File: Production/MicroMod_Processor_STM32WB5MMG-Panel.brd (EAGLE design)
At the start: 199.6 x 83.1 mm, 438 parts, among them J1 MICROMOD-2222, J10 MICROMOD-2222, J11 MICROMOD-2222, J12 MICROMOD-2222, J13 MICROMOD-2222, J14 MICROMOD-2222, J15 MICROMOD-2222, J16 MICROMOD-2222, J2 MICROMOD-2222, J3 MICROMOD-2222, J4 MICROMOD-2222, J5 MICROMOD-2222, J6 MICROMOD-2222, J7 MICROMOD-2222, J8 MICROMOD-2222, J9 MICROMOD-2222, Q1 20V/4.2A/52mΩ/1.4W, Q10 20V/4.2A/52mΩ/1.4W, Q11 20V/4.2A/52mΩ/1.4W, Q12 20V/4.2A/52mΩ/1.4W, Q13 20V/4.2A/52mΩ/1.4W, Q14 20V/4.2A/52mΩ/1.4W, Q15 20V/4.2A/52mΩ/1.4W, Q16 20V/4.2A/52mΩ/1.4W, Q2 20V/4.2A/52mΩ/1.4W, Q3 20V/4.2A/52mΩ/1.4W, Q4 20V/4.2A/52mΩ/1.4W, Q5 20V/4.2A/52mΩ/1.4W, Q6 20V/4.2A/52mΩ/1.4W, Q7 20V/4.2A/52mΩ/1.4W, Q8 20V/4.2A/52mΩ/1.4W, Q9 20V/4.2A/52mΩ/1.4W, U1 STM32WB5MMG, U10 STM32WB5MMG, U11 W25QXX128MBIT-6X5, U12 ESD Diode, U13 STM32WB5MMG, U14 W25QXX128MBIT-6X5, U15 ESD Diode, U16 STM32WB5MMG, U17 W25QXX128MBIT-6X5, U18 ESD Diode, U19 STM32WB5MMG, U2 W25QXX128MBIT-6X5, U20 W25QXX128MBIT-6X5, U21 ESD Diode, U22 STM32WB5MMG, U23 W25QXX128MBIT-6X5, U24 ESD Diode, U25 STM32WB5MMG, U26 W25QXX128MBIT-6X5, U27 ESD Diode, U28 STM32WB5MMG, U29 W25QXX128MBIT-6X5, U3 ESD Diode, U30 ESD Diode, U31 STM32WB5MMG, U32 W25QXX128MBIT-6X5, U33 ESD Diode, U34 STM32WB5MMG, U35 W25QXX128MBIT-6X5, U36 ESD Diode, U37 STM32WB5MMG, U38 W25QXX128MBIT-6X5, U39 ESD Diode, U4 STM32WB5MMG, U40 STM32WB5MMG, U41 W25QXX128MBIT-6X5, U42 ESD Diode, U43 STM32WB5MMG, U44 W25QXX128MBIT-6X5, U45 ESD Diode, U46 STM32WB5MMG, U47 W25QXX128MBIT-6X5, U48 ESD Diode, U5 W25QXX128MBIT-6X5, U6 ESD Diode, U7 STM32WB5MMG, U8 W25QXX128MBIT-6X5, U9 ESD Diode

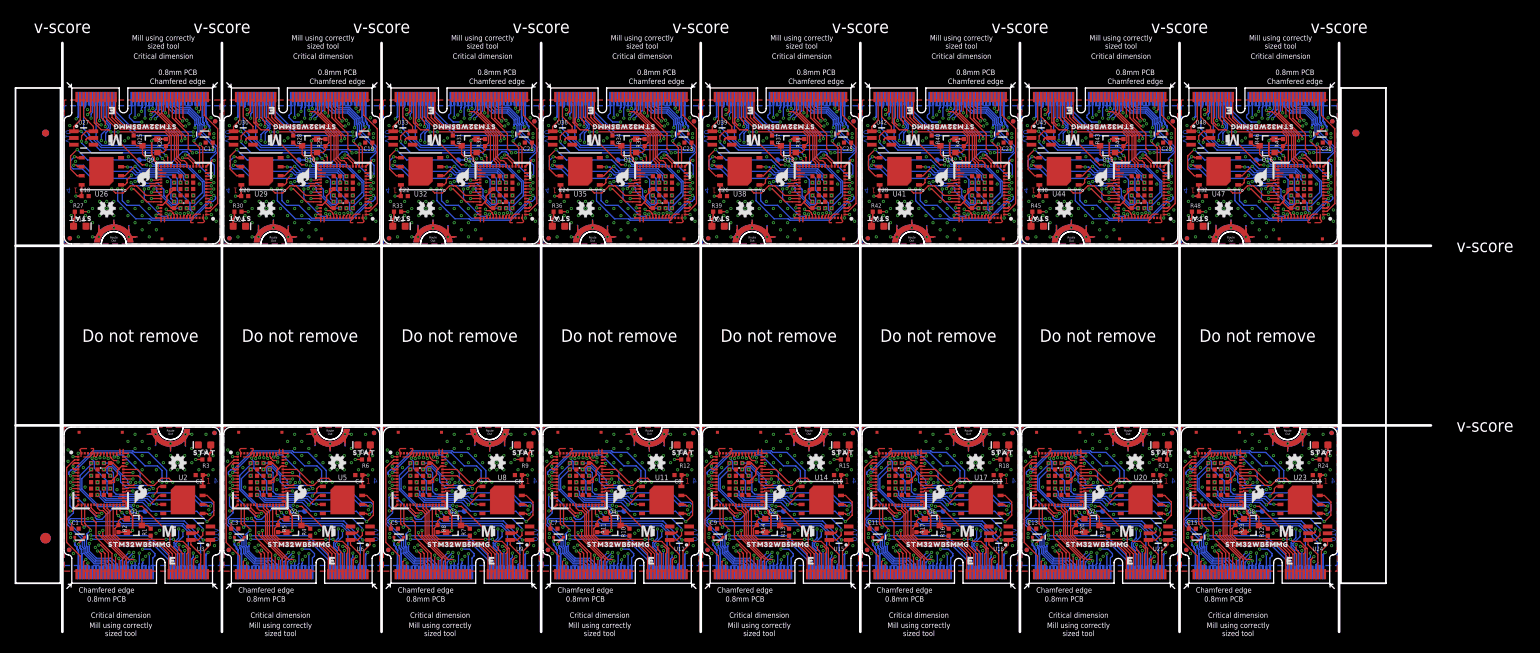
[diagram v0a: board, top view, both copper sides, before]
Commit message: v10 Update
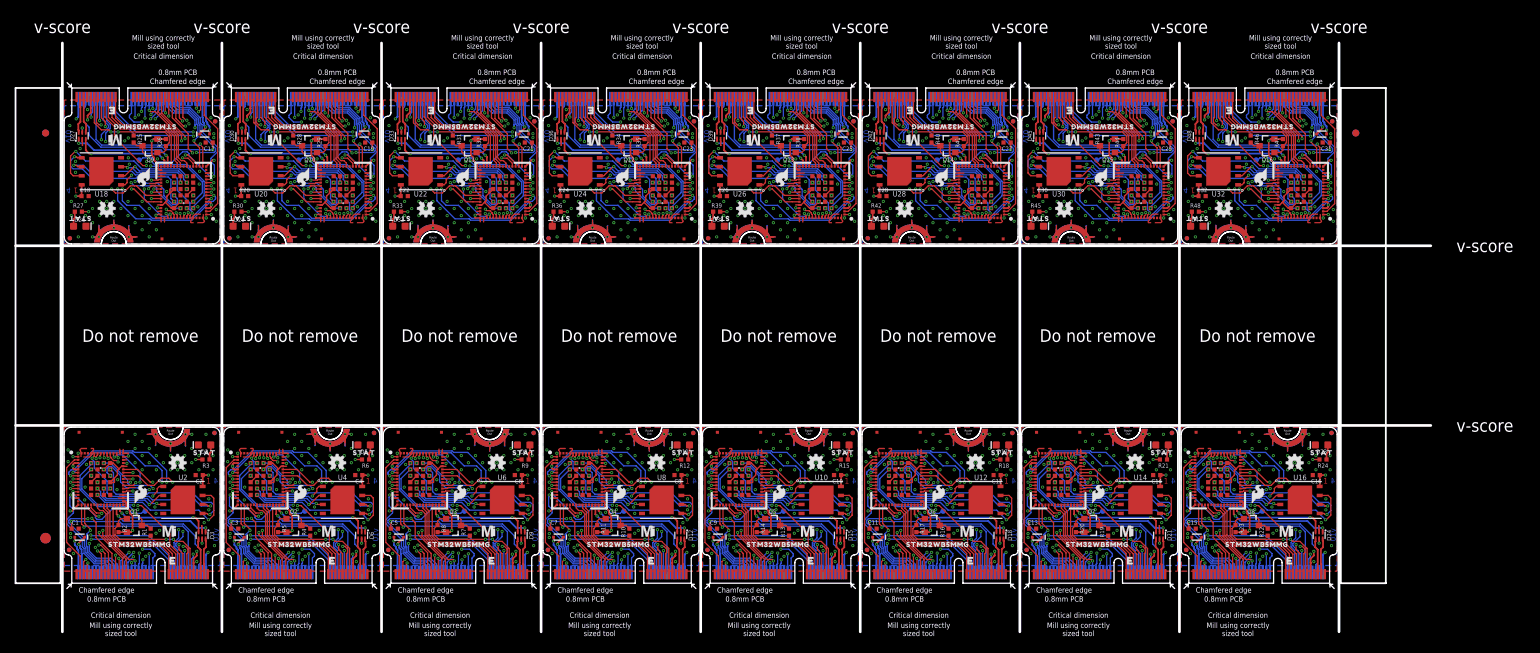
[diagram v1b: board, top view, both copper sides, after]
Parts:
- removed U33, U36, U39, U42, U45, U48: ESD Diode, SparkFun-DiscreteSemi:SOT-23-6
- removed U34, U37, U40, U43, U46: STM32WB5MMG, stm32wb5mmg:SIP-LGA86
- removed U35, U38, U41, U44, U47: W25QXX128MBIT-6X5, SparkFun-IC-Memory:WSON-8-6X5
- added D33, D36, D39, D42, D45, D48: PRTR5V0U2F, SparkFun-IC-Power:SOT886
- added D34, D37, D40, D43, D46: 120mA/40V/370mV, SparkFun-DiscreteSemi:SOD-523
- added D35, D38, D41, D44, D47: BLUE, SparkFun-LED:LED-0603
- D10, D16, D22, D28, D4: value BLUE -> 120mA/40V/370mV; device SparkFun-LED:LED-0603 -> SparkFun-DiscreteSemi:SOD-523
- D11, D17, D23, D29, D5: value 120mA/40V/370mV -> BLUE; device SparkFun-DiscreteSemi:SOD-523 -> SparkFun-LED:LED-0603
- D12, D18, D24, D30, D6: value BLUE -> PRTR5V0U2F; device SparkFun-LED:LED-0603 -> SparkFun-IC-Power:SOT886
- D15, D21, D27, D3, D9: value 120mA/40V/370mV -> PRTR5V0U2F; device SparkFun-DiscreteSemi:SOD-523 -> SparkFun-IC-Power:SOT886
- U10, U16, U22, U28, U4: value STM32WB5MMG -> W25QXX128MBIT-6X5; device stm32wb5mmg:SIP-LGA86 -> SparkFun-IC-Memory:WSON-8-6X5
- U11, U17, U23, U29, U5: value W25QXX128MBIT-6X5 -> STM32WB5MMG; device SparkFun-IC-Memory:WSON-8-6X5 -> stm32wb5mmg:SIP-LGA86
- U12, U18, U24, U30, U6: value ESD Diode -> W25QXX128MBIT-6X5; device SparkFun-DiscreteSemi:SOT-23-6 -> SparkFun-IC-Memory:WSON-8-6X5
- U15, U21, U27, U3, U9: value ESD Diode -> STM32WB5MMG; device SparkFun-DiscreteSemi:SOT-23-6 -> stm32wb5mmg:SIP-LGA86
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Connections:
- new net USBIN_N: D3.4, J1.5
- new net USBIN_N1: D6.4, J2.5
- new net USBIN_N10: D33.4, J11.5
- new net USBIN_N11: D36.4, J12.5
- new net USBIN_N12: D39.4, J13.5
- new net USBIN_N13: D42.4, J14.5
- new net USBIN_N14: D45.4, J15.5
- new net USBIN_N15: D48.4, J16.5
- new net USBIN_N2: D9.4, J3.5
- new net USBIN_N3: D12.4, J4.5
- new net USBIN_N4: D15.4, J5.5
- new net USBIN_N5: D18.4, J6.5
- new net USBIN_N6: D21.4, J7.5
- new net USBIN_N7: D24.4, J8.5
- new net USBIN_N8: D27.4, J9.5
- new net USBIN_N9: D30.4, J10.5
- new net USBIN_P: D3.6, J1.3
- new net USBIN_P1: D6.6, J2.3
- new net USBIN_P10: D33.6, J11.3
- new net USBIN_P11: D36.6, J12.3
- new net USBIN_P12: D39.6, J13.3
- new net USBIN_P13: D42.6, J14.3
- new net USBIN_P14: D45.6, J15.3
- new net USBIN_P15: D48.6, J16.3
- new net USBIN_P2: D9.6, J3.3
- new net USBIN_P3: D12.6, J4.3
- new net USBIN_P4: D15.6, J5.3
- new net USBIN_P5: D18.6, J6.3
- new net USBIN_P6: D21.6, J7.3
- new net USBIN_P7: D24.6, J8.3
- new net USBIN_P8: D27.6, J9.3
- new net USBIN_P9: D30.6, J10.3
- net !RESET!1: now also U3.10; no longer U4.10
- net !RESET!10: now also U21.10; no longer U31.10
- net !RESET!11: now also U23.10; no longer U34.10
- net !RESET!12: now also U25.10; no longer U37.10
- net !RESET!13: now also U27.10; no longer U40.10
- net !RESET!14: now also U29.10; no longer U43.10
- net !RESET!15: now also U31.10; no longer U46.10
- net !RESET!2: now also U5.10; no longer U7.10
- net !RESET!3: now also U7.10; no longer U10.10
- net !RESET!4: now also U9.10; no longer U13.10
- net !RESET!5: now also U11.10; no longer U16.10
- net !RESET!6: now also U13.10; no longer U19.10
- net !RESET!7: now also U15.10; no longer U22.10
- net !RESET!8: now also U17.10; no longer U25.10
- net !RESET!9: now also U19.10; no longer U28.10
- net 3.3V1: now also D4.A, U3.17, U3.32, U3.4, U3.6, U4.8; no longer D3.A, U4.17, U4.32, U4.4, U4.6, U5.8
- net 3.3V10: now also D31.A, U21.17, U21.32, U21.4, U21.6, U22.8; no longer D21.A, U31.17, U31.32, U31.4, U31.6, U32.8
- net 3.3V11: now also D34.A, U23.17, U23.32, U23.4, U23.6, U24.8; no longer D23.A, U34.17, U34.32, U34.4, U34.6, U35.8
- net 3.3V12: now also D37.A, U25.17, U25.32, U25.4, U25.6, U26.8; no longer D25.A, U37.17, U37.32, U37.4, U37.6, U38.8
- net 3.3V13: now also D40.A, U27.17, U27.32, U27.4, U27.6, U28.8; no longer D27.A, U40.17, U40.32, U40.4, U40.6, U41.8
- net 3.3V14: now also D43.A, U29.17, U29.32, U29.4, U29.6, U30.8; no longer D29.A, U43.17, U43.32, U43.4, U43.6, U44.8
- net 3.3V15: now also D46.A, U31.17, U31.32, U31.4, U31.6, U32.8; no longer D31.A, U46.17, U46.32, U46.4, U46.6, U47.8
- net 3.3V2: now also D7.A, U5.17, U5.32, U5.4, U5.6, U6.8; no longer D5.A, U7.17, U7.32, U7.4, U7.6, U8.8
- net 3.3V3: now also D10.A, U7.17, U7.32, U7.4, U7.6, U8.8; no longer D7.A, U10.17, U10.32, U10.4, U10.6, U11.8
- net 3.3V4: now also D13.A, U10.8, U9.17, U9.32, U9.4, U9.6; no longer D9.A, U13.17, U13.32, U13.4, U13.6, U14.8
- net 3.3V5: now also D16.A, U11.17, U11.32, U11.4, U11.6, U12.8; no longer D11.A, U16.17, U16.32, U16.4, U16.6, U17.8
- net 3.3V6: now also D19.A, U13.17, U13.32, U13.4, U13.6, U14.8; no longer D13.A, U19.17, U19.32, U19.4, U19.6, U20.8
- net 3.3V7: now also D22.A, U15.17, U15.32, U15.4, U15.6, U16.8; no longer D15.A, U22.17, U22.32, U22.4, U22.6, U23.8
- net 3.3V8: now also D25.A, U17.17, U17.32, U17.4, U17.6, U18.8; no longer D17.A, U25.17, U25.32, U25.4, U25.6, U26.8
- net 3.3V9: now also D28.A, U19.17, U19.32, U19.4, U19.6, U20.8; no longer D19.A, U28.17, U28.32, U28.4, U28.6, U29.8
- net A10: now also U11.8; no longer U16.8
- net A11: now also U11.7; no longer U16.7
- net A12: now also U13.8; no longer U19.8
- net A13: now also U13.7; no longer U19.7
- net A14: now also U15.8; no longer U22.8
- net A15: now also U15.7; no longer U22.7
- net A16: now also U17.8; no longer U25.8
- net A17: now also U17.7; no longer U25.7
- net A18: now also U19.8; no longer U28.8
- net A19: now also U19.7; no longer U28.7
- net A2: now also U3.8; no longer U4.8
- net A20: now also U21.8; no longer U31.8
- net A21: now also U21.7; no longer U31.7
- net A22: now also U23.8; no longer U34.8
- net A23: now also U23.7; no longer U34.7
- net A24: now also U25.8; no longer U37.8
- net A25: now also U25.7; no longer U37.7
- net A26: now also U27.8; no longer U40.8
- net A27: now also U27.7; no longer U40.7
- net A28: now also U29.8; no longer U43.8
- net A29: now also U29.7; no longer U43.7
- net A3: now also U3.7; no longer U4.7
- net A30: now also U31.8; no longer U46.8
- net A31: now also U31.7; no longer U46.7
- net A4: now also U5.8; no longer U7.8
- net A5: now also U5.7; no longer U7.7
- net A6: now also U7.8; no longer U10.8
- net A7: now also U7.7; no longer U10.7
- net A8: now also U9.8; no longer U13.8
- net A9: now also U9.7; no longer U13.7
- net AUD_BCLK1: now also U3.50; no longer U4.50
- net AUD_BCLK10: now also U21.50; no longer U31.50
- net AUD_BCLK11: now also U23.50; no longer U34.50
- net AUD_BCLK12: now also U25.50; no longer U37.50
- net AUD_BCLK13: now also U27.50; no longer U40.50
- net AUD_BCLK14: now also U29.50; no longer U43.50
- net AUD_BCLK15: now also U31.50; no longer U46.50
- net AUD_BCLK2: now also U5.50; no longer U7.50
- net AUD_BCLK3: now also U7.50; no longer U10.50
- net AUD_BCLK4: now also U9.50; no longer U13.50
- net AUD_BCLK5: now also U11.50; no longer U16.50
- net AUD_BCLK6: now also U13.50; no longer U19.50
- net AUD_BCLK7: now also U15.50; no longer U22.50
- net AUD_BCLK8: now also U17.50; no longer U25.50
- net AUD_BCLK9: now also U19.50; no longer U28.50
- net AUD_FSYNC1: now also U3.11; no longer U4.11
- net AUD_FSYNC10: now also U21.11; no longer U31.11
- net AUD_FSYNC11: now also U23.11; no longer U34.11
- net AUD_FSYNC12: now also U25.11; no longer U37.11
- net AUD_FSYNC13: now also U27.11; no longer U40.11
- net AUD_FSYNC14: now also U29.11; no longer U43.11
- net AUD_FSYNC15: now also U31.11; no longer U46.11
- net AUD_FSYNC2: now also U5.11; no longer U7.11
- net AUD_FSYNC3: now also U7.11; no longer U10.11
- net AUD_FSYNC4: now also U9.11; no longer U13.11
- net AUD_FSYNC5: now also U11.11; no longer U16.11
- net AUD_FSYNC6: now also U13.11; no longer U19.11
- net AUD_FSYNC7: now also U15.11; no longer U22.11
- net AUD_FSYNC8: now also U17.11; no longer U25.11
- net AUD_FSYNC9: now also U19.11; no longer U28.11
- net AUD_I2S_IN1: now also U3.19; no longer U4.19
- net AUD_I2S_IN10: now also U21.19; no longer U31.19
- net AUD_I2S_IN11: now also U23.19; no longer U34.19
- net AUD_I2S_IN12: now also U25.19; no longer U37.19
- net AUD_I2S_IN13: now also U27.19; no longer U40.19
- net AUD_I2S_IN14: now also U29.19; no longer U43.19
- net AUD_I2S_IN15: now also U31.19; no longer U46.19
- net AUD_I2S_IN2: now also U5.19; no longer U7.19
- net AUD_I2S_IN3: now also U7.19; no longer U10.19
- net AUD_I2S_IN4: now also U9.19; no longer U13.19
- net AUD_I2S_IN5: now also U11.19; no longer U16.19
- net AUD_I2S_IN6: now also U13.19; no longer U19.19
- net AUD_I2S_IN7: now also U15.19; no longer U22.19
- net AUD_I2S_IN8: now also U17.19; no longer U25.19
- net AUD_I2S_IN9: now also U19.19; no longer U28.19
- net AUD_I2S_OUT1: now also U3.38; no longer U4.38
- net AUD_I2S_OUT10: now also U21.38; no longer U31.38
- net AUD_I2S_OUT11: now also U23.38; no longer U34.38
- net AUD_I2S_OUT12: now also U25.38; no longer U37.38
- net AUD_I2S_OUT13: now also U27.38; no longer U40.38
- net AUD_I2S_OUT14: now also U29.38; no longer U43.38
- net AUD_I2S_OUT15: now also U31.38; no longer U46.38
- net AUD_I2S_OUT2: now also U5.38; no longer U7.38
- net AUD_I2S_OUT3: now also U7.38; no longer U10.38
- net AUD_I2S_OUT4: now also U9.38; no longer U13.38
- net AUD_I2S_OUT5: now also U11.38; no longer U16.38
- net AUD_I2S_OUT6: now also U13.38; no longer U19.38
- net AUD_I2S_OUT7: now also U15.38; no longer U22.38
- net AUD_I2S_OUT8: now also U17.38; no longer U25.38
- net AUD_I2S_OUT9: now also U19.38; no longer U28.38
- net AUD_MCLK1: now also U3.14; no longer U4.14
- net AUD_MCLK10: now also U21.14; no longer U31.14
- net AUD_MCLK11: now also U23.14; no longer U34.14
- net AUD_MCLK12: now also U25.14; no longer U37.14
- net AUD_MCLK13: now also U27.14; no longer U40.14
- net AUD_MCLK14: now also U29.14; no longer U43.14
- net AUD_MCLK15: now also U31.14; no longer U46.14
- net AUD_MCLK2: now also U5.14; no longer U7.14
- net AUD_MCLK3: now also U7.14; no longer U10.14
- net AUD_MCLK4: now also U9.14; no longer U13.14
- net AUD_MCLK5: now also U11.14; no longer U16.14
- net AUD_MCLK6: now also U13.14; no longer U19.14
- net AUD_MCLK7: now also U15.14; no longer U22.14
- net AUD_MCLK8: now also U17.14; no longer U25.14
- net AUD_MCLK9: now also U19.14; no longer U28.14
- net BATT_VIN1: now also U3.49; no longer U4.49
- net BATT_VIN10: now also U21.49; no longer U31.49
- net BATT_VIN11: now also U23.49; no longer U34.49
- net BATT_VIN12: now also U25.49; no longer U37.49
- net BATT_VIN13: now also U27.49; no longer U40.49
- net BATT_VIN14: now also U29.49; no longer U43.49
- net BATT_VIN15: now also U31.49; no longer U46.49
- net BATT_VIN2: now also U5.49; no longer U7.49
- net BATT_VIN3: now also U7.49; no longer U10.49
- net BATT_VIN4: now also U9.49; no longer U13.49
- net BATT_VIN5: now also U11.49; no longer U16.49
- net BATT_VIN6: now also U13.49; no longer U19.49
- net BATT_VIN7: now also U15.49; no longer U22.49
- net BATT_VIN8: now also U17.49; no longer U25.49
- net BATT_VIN9: now also U19.49; no longer U28.49
- net BOOT1: now also U3.13; no longer U4.13
- net BOOT10: now also U21.13; no longer U31.13
- net BOOT11: now also U23.13; no longer U34.13
- net BOOT12: now also U25.13; no longer U37.13
- net BOOT13: now also U27.13; no longer U40.13
- net BOOT14: now also U29.13; no longer U43.13
- net BOOT15: now also U31.13; no longer U46.13
- net BOOT2: now also U5.13; no longer U7.13
- net BOOT3: now also U7.13; no longer U10.13
- net BOOT4: now also U9.13; no longer U13.13
- net BOOT5: now also U11.13; no longer U16.13
- net BOOT6: now also U13.13; no longer U19.13
- net BOOT7: now also U15.13; no longer U22.13
- net BOOT8: now also U17.13; no longer U25.13
- net BOOT9: now also U19.13; no longer U28.13
- net GND: now also D3.2; no longer U3.2
- net GND10: now also D17.C, D18.2, U11.16, U11.22, U11.24, U11.27, U11.31, U11.33, U11.34, U11.36, U11.43, U11.44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; no longer D12.C, U16.16, U16.22, U16.24, U16.27, U16.31, U16.33, U16.34, U16.36, U16.43, U16.44, U16.45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
- net GND12: now also D20.C, D21.2, U13.16, U13.22, U13.24, U13.27, U13.31, U13.33, U13.34, U13.36, U13.43, U13.44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; no longer D14.C, U19.16, U19.22, U19.24, U19.27, U19.31, U19.33, U19.34, U19.36, U19.43, U19.44, U19.45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
- net GND14: now also D23.C, D24.2, U15.16, U15.22, U15.24, U15.27, U15.31, U15.33, U15.34, U15.36, U15.43, U15.44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; no longer D16.C, U22.16, U22.22, U22.24, U22.27, U22.31, U22.33, U22.34, U22.36, U22.43, U22.44, U22.45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
- net GND16: now also D26.C, D27.2, U17.16, U17.22, U17.24, U17.27, U17.31, U17.33, U17.34, U17.36, U17.43, U17.44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; no longer D18.C, U25.16, U25.22, U25.24, U25.27, U25.31, U25.33, U25.34, U25.36, U25.43, U25.44, U25.45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
- net GND18: now also D29.C, D30.2, U19.16, U19.22, U19.24, U19.27, U19.31, U19.33, U19.34, U19.36, U19.43, U19.44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; no longer D20.C, U28.16, U28.22, U28.24, U28.27, U28.31, U28.33, U28.34, U28.36, U28.43, U28.44, U28.45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
- net GND2: now also D5.C, D6.2, U3.16, U3.22, U3.24, U3.27, U3.31, U3.33, U3.34, U3.36, U3.43, U3.44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; no longer D4.C, U4.16, U4.22, U4.24, U4.27, U4.31, U4.33, U4.34, U4.36, U4.43, U4.44, U4.45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
- net GND20: now also D32.C, D33.2, U21.16, U21.22, U21.24, U21.27, U21.31, U21.33, U21.34, U21.36, U21.43, U21.44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; no longer D22.C, U31.16, U31.22, U31.24, U31.27, U31.31, U31.33, U31.34, U31.36, U31.43, U31.44, U31.45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
- net GND22: now also D35.C, D36.2, U23.16, U23.22, U23.24, U23.27, U23.31, U23.33, U23.34, U23.36, U23.43, U23.44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; no longer D24.C, U34.16, U34.22, U34.24, U34.27, U34.31, U34.33, U34.34, U34.36, U34.43, U34.44, U34.45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
- net GND24: now also D38.C, D39.2, U25.16, U25.22, U25.24, U25.27, U25.31, U25.33, U25.34, U25.36, U25.43, U25.44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; no longer D26.C, U37.16, U37.22, U37.24, U37.27, U37.31, U37.33, U37.34, U37.36, U37.43, U37.44, U37.45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
- net GND26: now also D41.C, D42.2, U27.16, U27.22, U27.24, U27.27, U27.31, U27.33, U27.34, U27.36, U27.43, U27.44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; no longer D28.C, U40.16, U40.22, U40.24, U40.27, U40.31, U40.33, U40.34, U40.36, U40.43, U40.44, U40.45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
- net GND28: now also D44.C, D45.2, U29.16, U29.22, U29.24, U29.27, U29.31, U29.33, U29.34, U29.36, U29.43, U29.44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; no longer D30.C, U43.16, U43.22, U43.24, U43.27, U43.31, U43.33, U43.34, U43.36, U43.43, U43.44, U43.45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
- net GND30: now also D47.C, D48.2, U31.16, U31.22, U31.24, U31.27, U31.31, U31.33, U31.34, U31.36, U31.43, U31.44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; no longer D32.C, U46.16, U46.22, U46.24, U46.27, U46.31, U46.33, U46.34, U46.36, U46.43, U46.44, U46.45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
- net GND4: now also D8.C, D9.2, U5.16, U5.22, U5.24, U5.27, U5.31, U5.33, U5.34, U5.36, U5.43, U5.44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; no longer D6.C, U7.16, U7.22, U7.24, U7.27, U7.31, U7.33, U7.34, U7.36, U7.43, U7.44, U7.45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
- net GND6: now also D11.C, D12.2, U7.16, U7.22, U7.24, U7.27, U7.31, U7.33, U7.34, U7.36, U7.43, U7.44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; no longer D8.C, U10.16, U10.22, U10.24, U10.27, U10.31, U10.33, U10.34, U10.36, U10.43, U10.44, U10.45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
- net GND8: now also D14.C, D15.2, U10.4, U9.16, U9.22, U9.24, U9.27, U9.31, U9.33, U9.34, U9.36, U9.43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; no longer D10.C, U13.16, U13.22, U13.24, U13.27, U13.31, U13.33, U13.34, U13.36, U13.43, U13.44, U13.45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
- net I2C1_INT1: now also U3.2; no longer U4.2
- net I2C1_INT10: now also U21.2; no longer U31.2
- net I2C1_INT11: now also U23.2; no longer U34.2
- net I2C1_INT12: now also U25.2; no longer U37.2
- net I2C1_INT13: now also U27.2; no longer U40.2
- net I2C1_INT14: now also U29.2; no longer U43.2
- net I2C1_INT15: now also U31.2; no longer U46.2
- net I2C1_INT2: now also U5.2; no longer U7.2
- net I2C1_INT3: now also U7.2; no longer U10.2
- net I2C1_INT4: now also U9.2; no longer U13.2
- net I2C1_INT5: now also U11.2; no longer U16.2
- net I2C1_INT6: now also U13.2; no longer U19.2
- net I2C1_INT7: now also U15.2; no longer U22.2
- net I2C1_INT8: now also U17.2; no longer U25.2
- net I2C1_INT9: now also U19.2; no longer U28.2
- net I2C1_SCL1: now also U3.39; no longer U4.39
- net I2C1_SCL10: now also U21.39; no longer U31.39
- net I2C1_SCL11: now also U23.39; no longer U34.39
- net I2C1_SCL12: now also U25.39; no longer U37.39
- net I2C1_SCL13: now also U27.39; no longer U40.39
- net I2C1_SCL14: now also U29.39; no longer U43.39
- net I2C1_SCL15: now also U31.39; no longer U46.39
- net I2C1_SCL2: now also U5.39; no longer U7.39
- net I2C1_SCL3: now also U7.39; no longer U10.39
- net I2C1_SCL4: now also U9.39; no longer U13.39
- net I2C1_SCL5: now also U11.39; no longer U16.39
- net I2C1_SCL6: now also U13.39; no longer U19.39
- net I2C1_SCL7: now also U15.39; no longer U22.39
- net I2C1_SCL8: now also U17.39; no longer U25.39
- net I2C1_SCL9: now also U19.39; no longer U28.39
- net I2C1_SDA1: now also U3.18; no longer U4.18
- net I2C1_SDA10: now also U21.18; no longer U31.18
- net I2C1_SDA11: now also U23.18; no longer U34.18
- net I2C1_SDA12: now also U25.18; no longer U37.18
- net I2C1_SDA13: now also U27.18; no longer U40.18
- net I2C1_SDA14: now also U29.18; no longer U43.18
- net I2C1_SDA15: now also U31.18; no longer U46.18
- net I2C1_SDA2: now also U5.18; no longer U7.18
- net I2C1_SDA3: now also U7.18; no longer U10.18
- net I2C1_SDA4: now also U9.18; no longer U13.18
- net I2C1_SDA5: now also U11.18; no longer U16.18
- net I2C1_SDA6: now also U13.18; no longer U19.18
- net I2C1_SDA7: now also U15.18; no longer U22.18
- net I2C1_SDA8: now also U17.18; no longer U25.18
- net I2C1_SDA9: now also U19.18; no longer U28.18
- net I2C3_SCL10: now also U19.35; no longer U28.35
- net I2C3_SCL11: now also U21.35; no longer U31.35
- net I2C3_SCL12: now also U23.35; no longer U34.35
- net I2C3_SCL13: now also U25.35; no longer U37.35
- net I2C3_SCL14: now also U27.35; no longer U40.35
- net I2C3_SCL15: now also U29.35; no longer U43.35
- net I2C3_SCL16: now also U31.35; no longer U46.35
- net I2C3_SCL2: now also U3.35; no longer U4.35
- net I2C3_SCL3: now also U5.35; no longer U7.35
- net I2C3_SCL4: now also U7.35; no longer U10.35
- net I2C3_SCL5: now also U9.35; no longer U13.35
- net I2C3_SCL6: now also U11.35; no longer U16.35
- net I2C3_SCL7: now also U13.35; no longer U19.35
- net I2C3_SCL8: now also U15.35; no longer U22.35
- net I2C3_SCL9: now also U17.35; no longer U25.35
- net I2C3_SDA10: now also U19.37; no longer U28.37
- net I2C3_SDA11: now also U21.37; no longer U31.37
- net I2C3_SDA12: now also U23.37; no longer U34.37
- net I2C3_SDA13: now also U25.37; no longer U37.37
- net I2C3_SDA14: now also U27.37; no longer U40.37
- net I2C3_SDA15: now also U29.37; no longer U43.37
- net I2C3_SDA16: now also U31.37; no longer U46.37
- net I2C3_SDA2: now also U3.37; no longer U4.37
- net I2C3_SDA3: now also U5.37; no longer U7.37
- net I2C3_SDA4: now also U7.37; no longer U10.37
- net I2C3_SDA5: now also U9.37; no longer U13.37
- net I2C3_SDA6: now also U11.37; no longer U16.37
- net I2C3_SDA7: now also U13.37; no longer U19.37
- net I2C3_SDA8: now also U15.37; no longer U22.37
- net I2C3_SDA9: now also U17.37; no longer U25.37
- net LP_RX2/DEV_TX1: now also U3.12; no longer U4.12
- net LP_RX2/DEV_TX10: now also U19.12; no longer U28.12
- net LP_RX2/DEV_TX11: now also U21.12; no longer U31.12
- net LP_RX2/DEV_TX12: now also U23.12; no longer U34.12
- net LP_RX2/DEV_TX13: now also U25.12; no longer U37.12
- net LP_RX2/DEV_TX14: now also U27.12; no longer U40.12
- net LP_RX2/DEV_TX15: now also U29.12; no longer U43.12
- net LP_RX2/DEV_TX16: now also U31.12; no longer U46.12
- net LP_RX2/DEV_TX3: now also U5.12; no longer U7.12
- net LP_RX2/DEV_TX4: now also U7.12; no longer U10.12
- net LP_RX2/DEV_TX5: now also U9.12; no longer U13.12
- net LP_RX2/DEV_TX6: now also U11.12; no longer U16.12
- net LP_RX2/DEV_TX7: now also U13.12; no longer U19.12
- net LP_RX2/DEV_TX8: now also U15.12; no longer U22.12
- net LP_RX2/DEV_TX9: now also U17.12; no longer U25.12
- net LP_TX2/DEV_RX1: now also U3.9; no longer U4.9
- net LP_TX2/DEV_RX10: now also U19.9; no longer U28.9
- net LP_TX2/DEV_RX11: now also U21.9; no longer U31.9
- net LP_TX2/DEV_RX12: now also U23.9; no longer U34.9
- net LP_TX2/DEV_RX13: now also U25.9; no longer U37.9
- net LP_TX2/DEV_RX14: now also U27.9; no longer U40.9
- net LP_TX2/DEV_RX15: now also U29.9; no longer U43.9
- net LP_TX2/DEV_RX16: now also U31.9; no longer U46.9
- net LP_TX2/DEV_RX3: now also U5.9; no longer U7.9
- net LP_TX2/DEV_RX4: now also U7.9; no longer U10.9
- net LP_TX2/DEV_RX5: now also U9.9; no longer U13.9
- net LP_TX2/DEV_RX6: now also U11.9; no longer U16.9
- net LP_TX2/DEV_RX7: now also U13.9; no longer U19.9
- net LP_TX2/DEV_RX8: now also U15.9; no longer U22.9
- net LP_TX2/DEV_RX9: now also U17.9; no longer U25.9
- net N$10: now also D15.5; no longer U15.5
- net N$11: now also D17.A; no longer D12.A
- net N$12: now also D18.5; no longer U18.5
- net N$13: now also D20.A; no longer D14.A
- net N$14: now also D21.5; no longer U21.5
- net N$15: now also D23.A; no longer D16.A
- net N$16: now also D24.5; no longer U24.5
- net N$17: now also D26.A; no longer D18.A
- net N$18: now also D27.5; no longer U27.5
- net N$19: now also D29.A; no longer D20.A
- net N$2: now also D5.A, R6.1; no longer J1.9, U3.5
- net N$20: now also D30.5; no longer U30.5
- net N$21: now also D32.A; no longer D22.A
- net N$22: now also D33.5; no longer U33.5
- net N$23: now also D35.A; no longer D24.A
- net N$24: now also D36.5; no longer U36.5
- net N$25: now also D38.A; no longer D26.A
- net N$26: now also D39.5; no longer U39.5
- net N$27: now also D41.A; no longer D28.A
- net N$28: now also D42.5; no longer U42.5
- net N$29: now also D44.A; no longer D30.A
- net N$3: now also D6.5, J2.9; no longer D4.A, R6.1
- net N$30: now also D45.5; no longer U45.5
- net N$31: now also D47.A; no longer D32.A
- net N$32: now also D48.5; no longer U48.5
- net N$4: now also D3.5, J1.9; no longer J2.9, U6.5
- net N$5: now also D8.A; no longer D6.A
- net N$6: now also D9.5; no longer U9.5
- net N$7: now also D11.A; no longer D8.A
- net N$8: now also D12.5; no longer U12.5
- net N$9: now also D14.A; no longer D10.A
- net PA0/G1: now also U3.3; no longer U4.3
- net PA0/G10: now also U19.3; no longer U28.3
- net PA0/G11: now also U21.3; no longer U31.3
- net PA0/G12: now also U23.3; no longer U34.3
- net PA0/G13: now also U25.3; no longer U37.3
- net PA0/G14: now also U27.3; no longer U40.3
- net PA0/G15: now also U29.3; no longer U43.3
- net PA0/G16: now also U31.3; no longer U46.3
- net PA0/G2: now also U5.3; no longer U7.3
- net PA0/G3: now also U7.3; no longer U10.3
- net PA0/G4: now also U9.3; no longer U13.3
- net PA0/G6: now also U11.3; no longer U16.3
- net PA0/G7: now also U13.3; no longer U19.3
- net PA0/G8: now also U15.3; no longer U22.3
- net PA0/G9: now also U17.3; no longer U25.3
- net PC11/G10: now also U19.23; no longer U28.23
- net PC11/G11: now also U21.23; no longer U31.23
- net PC11/G12: now also U23.23; no longer U34.23
- net PC11/G13: now also U25.23; no longer U37.23
- net PC11/G14: now also U27.23; no longer U40.23
- net PC11/G15: now also U29.23; no longer U43.23
- net PC11/G16: now also U31.23; no longer U46.23
- net PC11/G2: now also U3.23; no longer U4.23
- net PC11/G3: now also U5.23; no longer U7.23
- net PC11/G4: now also U7.23; no longer U10.23
- net PC11/G5: now also U9.23; no longer U13.23
- net PC11/G6: now also U11.23; no longer U16.23
- net PC11/G7: now also U13.23; no longer U19.23
- net PC11/G8: now also U15.23; no longer U22.23
- net PC11/G9: now also U17.23; no longer U25.23
- net PC13/G1: now also U3.40; no longer U4.40
- net PC13/G10: now also U19.40; no longer U28.40
- net PC13/G11: now also U21.40; no longer U31.40
- net PC13/G12: now also U23.40; no longer U34.40
- net PC13/G13: now also U25.40; no longer U37.40
- net PC13/G14: now also U27.40; no longer U40.40
- net PC13/G15: now also U29.40; no longer U43.40
- net PC13/G16: now also U31.40; no longer U46.40
- net PC13/G3: now also U5.40; no longer U7.40
- net PC13/G4: now also U7.40; no longer U10.40
- net PC13/G5: now also U9.40; no longer U13.40
- net PC13/G6: now also U11.40; no longer U16.40
- net PC13/G7: now also U13.40; no longer U19.40
- net PC13/G8: now also U15.40; no longer U22.40
- net PC13/G9: now also U17.40; no longer U25.40
- net PD8/G1: now also U3.75; no longer U4.75
- net PD8/G10: now also U19.75; no longer U28.75
- net PD8/G11: now also U21.75; no longer U31.75
- net PD8/G12: now also U23.75; no longer U34.75
- net PD8/G13: now also U25.75; no longer U37.75
- net PD8/G14: now also U27.75; no longer U40.75
- net PD8/G15: now also U29.75; no longer U43.75
- net PD8/G16: now also U31.75; no longer U46.75
- net PD8/G2: now also U5.75; no longer U7.75
- net PD8/G4: now also U7.75; no longer U10.75
- net PD8/G5: now also U9.75; no longer U13.75
- net PD8/G6: now also U11.75; no longer U16.75
- net PD8/G7: now also U13.75; no longer U19.75
- net PD8/G8: now also U15.75; no longer U22.75
- net PD8/G9: now also U17.75; no longer U25.75
- net PE3/G1: now also U3.72; no longer U4.72
- net PE3/G10: now also U19.72; no longer U28.72
- net PE3/G11: now also U21.72; no longer U31.72
- net PE3/G12: now also U23.72; no longer U34.72
- net PE3/G13: now also U25.72; no longer U37.72
- net PE3/G14: now also U27.72; no longer U40.72
- net PE3/G15: now also U29.72; no longer U43.72
- net PE3/G16: now also U31.72; no longer U46.72
- net PE3/G2: now also U5.72; no longer U7.72
- net PE3/G3: now also U7.72; no longer U10.72
- net PE3/G5: now also U9.72; no longer U13.72
- net PE3/G6: now also U11.72; no longer U16.72
- net PE3/G7: now also U13.72; no longer U19.72
- net PE3/G8: now also U15.72; no longer U22.72
- net PE3/G9: now also U17.72; no longer U25.72
- net PE4/G1: now also U3.42; no longer U4.42
- net PE4/G10: now also U21.42; no longer U31.42
- net PE4/G11: now also U23.42; no longer U34.42
- net PE4/G12: now also U25.42; no longer U37.42
- net PE4/G13: now also U27.42; no longer U40.42
- net PE4/G14: now also U29.42; no longer U43.42
- net PE4/G15: now also U31.42; no longer U46.42
- net PE4/G2: now also U5.42; no longer U7.42
- net PE4/G3: now also U7.42; no longer U10.42
- net PE4/G4: now also U9.42; no longer U13.42
- net PE4/G5: now also U11.42; no longer U16.42
- net PE4/G6: now also U13.42; no longer U19.42
- net PE4/G7: now also U15.42; no longer U22.42
- net PE4/G8: now also U17.42; no longer U25.42
- net PE4/G9: now also U19.42; no longer U28.42
- net PH0/G1: now also U3.61; no longer U4.61
- net PH0/G10: now also U19.61; no longer U28.61
- net PH0/G11: now also U21.61; no longer U31.61
- net PH0/G12: now also U23.61; no longer U34.61
- net PH0/G13: now also U25.61; no longer U37.61
- net PH0/G14: now also U27.61; no longer U40.61
- net PH0/G15: now also U29.61; no longer U43.61
- net PH0/G16: now also U31.61; no longer U46.61
- net PH0/G2: now also U5.61; no longer U7.61
- net PH0/G3: now also U7.61; no longer U10.61
- net PH0/G4: now also U9.61; no longer U13.61
- net PH0/G5: now also U11.61; no longer U16.61
- net PH0/G6: now also U13.61; no longer U19.61
- net PH0/G8: now also U15.61; no longer U22.61
- net PH0/G9: now also U17.61; no longer U25.61
- net PH1/G1: now also U3.62; no longer U4.62
- net PH1/G10: now also U19.62; no longer U28.62
- net PH1/G11: now also U21.62; no longer U31.62
- net PH1/G12: now also U23.62; no longer U34.62
- net PH1/G13: now also U25.62; no longer U37.62
- net PH1/G14: now also U27.62; no longer U40.62
- net PH1/G15: now also U29.62; no longer U43.62
- net PH1/G16: now also U31.62; no longer U46.62
- net PH1/G2: now also U5.62; no longer U7.62
- net PH1/G3: now also U7.62; no longer U10.62
- net PH1/G4: now also U9.62; no longer U13.62
- net PH1/G5: now also U11.62; no longer U16.62
- net PH1/G7: now also U13.62; no longer U19.62
- net PH1/G8: now also U15.62; no longer U22.62
- net PH1/G9: now also U17.62; no longer U25.62
- net PWM10: now also U11.63; no longer U16.63
- net PWM11: now also U11.76; no longer U16.76
- net PWM12: now also U13.63; no longer U19.63
- net PWM13: now also U13.76; no longer U19.76
- net PWM14: now also U15.63; no longer U22.63
- net PWM15: now also U15.76; no longer U22.76
- net PWM16: now also U17.63; no longer U25.63
- net PWM17: now also U17.76; no longer U25.76
- net PWM18: now also U19.63; no longer U28.63
- net PWM19: now also U19.76; no longer U28.76
- net PWM2: now also U3.63; no longer U4.63
- net PWM20: now also U21.63; no longer U31.63
- net PWM21: now also U21.76; no longer U31.76
- net PWM22: now also U23.63; no longer U34.63
- net PWM23: now also U23.76; no longer U34.76
- net PWM24: now also U25.63; no longer U37.63
- net PWM25: now also U25.76; no longer U37.76
- net PWM26: now also U27.63; no longer U40.63
- net PWM27: now also U27.76; no longer U40.76
- net PWM28: now also U29.63; no longer U43.63
- net PWM29: now also U29.76; no longer U43.76
- net PWM3: now also U3.76; no longer U4.76
- net PWM30: now also U31.63; no longer U46.63
- net PWM31: now also U31.76; no longer U46.76
- net PWM4: now also U5.63; no longer U7.63
- net PWM5: now also U5.76; no longer U7.76
- net PWM6: now also U7.63; no longer U10.63
- net PWM7: now also U7.76; no longer U10.76
- net PWM8: now also U9.63; no longer U13.63
- net PWM9: now also U9.76; no longer U13.76
- net QSPI_!CS!1: now also U3.70, U4.1; no longer U4.70, U5.1
- net QSPI_!CS!10: now also U21.70, U22.1; no longer U31.70, U32.1
- net QSPI_!CS!11: now also U23.70, U24.1; no longer U34.70, U35.1
- net QSPI_!CS!12: now also U25.70, U26.1; no longer U37.70, U38.1
- net QSPI_!CS!13: now also U27.70, U28.1; no longer U40.70, U41.1
- net QSPI_!CS!14: now also U29.70, U30.1; no longer U43.70, U44.1
- net QSPI_!CS!15: now also U31.70, U32.1; no longer U46.70, U47.1
- net QSPI_!CS!2: now also U5.70, U6.1; no longer U7.70, U8.1
- net QSPI_!CS!3: now also U7.70, U8.1; no longer U10.70, U11.1
- net QSPI_!CS!4: now also U10.1, U9.70; no longer U13.70, U14.1
- net QSPI_!CS!5: now also U11.70, U12.1; no longer U16.70, U17.1
- net QSPI_!CS!6: now also U13.70, U14.1; no longer U19.70, U20.1
- net QSPI_!CS!7: now also U15.70, U16.1; no longer U22.70, U23.1
- net QSPI_!CS!8: now also U17.70, U18.1; no longer U25.70, U26.1
- net QSPI_!CS!9: now also U19.70, U20.1; no longer U28.70, U29.1
- net QSPI_CLK1: now also U3.56, U4.6; no longer U4.56, U5.6
- net QSPI_CLK10: now also U21.56, U22.6; no longer U31.56, U32.6
- net QSPI_CLK11: now also U23.56, U24.6; no longer U34.56, U35.6
- net QSPI_CLK12: now also U25.56, U26.6; no longer U37.56, U38.6
- net QSPI_CLK13: now also U27.56, U28.6; no longer U40.56, U41.6
- net QSPI_CLK14: now also U29.56, U30.6; no longer U43.56, U44.6
- net QSPI_CLK15: now also U31.56, U32.6; no longer U46.56, U47.6
- net QSPI_CLK2: now also U5.56, U6.6; no longer U7.56, U8.6
- net QSPI_CLK3: now also U7.56, U8.6; no longer U10.56, U11.6
- net QSPI_CLK4: now also U10.6, U9.56; no longer U13.56, U14.6
- net QSPI_CLK5: now also U11.56, U12.6; no longer U16.56, U17.6
- net QSPI_CLK6: now also U13.56, U14.6; no longer U19.56, U20.6
- net QSPI_CLK7: now also U15.56, U16.6; no longer U22.56, U23.6
- net QSPI_CLK8: now also U17.56, U18.6; no longer U25.56, U26.6
- net QSPI_CLK9: now also U19.56, U20.6; no longer U28.56, U29.6
- net QSPI_IO10: now also U5.81, U6.3; no longer U7.81, U8.3
- net QSPI_IO11: now also U5.67, U6.7; no longer U7.67, U8.7
- net QSPI_IO12: now also U7.73, U8.5; no longer U10.73, U11.5
- net QSPI_IO13: now also U7.80, U8.2; no longer U10.80, U11.2
- net QSPI_IO14: now also U7.81, U8.3; no longer U10.81, U11.3
- net QSPI_IO15: now also U7.67, U8.7; no longer U10.67, U11.7
- net QSPI_IO16: now also U10.5, U9.73; no longer U13.73, U14.5
- net QSPI_IO17: now also U10.2, U9.80; no longer U13.80, U14.2
- net QSPI_IO18: now also U10.3, U9.81; no longer U13.81, U14.3
- net QSPI_IO19: now also U10.7, U9.67; no longer U13.67, U14.7
- net QSPI_IO20: now also U11.73, U12.5; no longer U16.73, U17.5
- net QSPI_IO21: now also U11.80, U12.2; no longer U16.80, U17.2
- net QSPI_IO22: now also U11.81, U12.3; no longer U16.81, U17.3
- net QSPI_IO23: now also U11.67, U12.7; no longer U16.67, U17.7
- net QSPI_IO24: now also U13.73, U14.5; no longer U19.73, U20.5
- net QSPI_IO25: now also U13.80, U14.2; no longer U19.80, U20.2
- net QSPI_IO26: now also U13.81, U14.3; no longer U19.81, U20.3
- net QSPI_IO27: now also U13.67, U14.7; no longer U19.67, U20.7
- net QSPI_IO28: now also U15.73, U16.5; no longer U22.73, U23.5
- net QSPI_IO29: now also U15.80, U16.2; no longer U22.80, U23.2
- net QSPI_IO30: now also U15.81, U16.3; no longer U22.81, U23.3
- net QSPI_IO31: now also U15.67, U16.7; no longer U22.67, U23.7
- net QSPI_IO32: now also U17.73, U18.5; no longer U25.73, U26.5
- net QSPI_IO33: now also U17.80, U18.2; no longer U25.80, U26.2
- net QSPI_IO34: now also U17.81, U18.3; no longer U25.81, U26.3
- net QSPI_IO35: now also U17.67, U18.7; no longer U25.67, U26.7
- net QSPI_IO36: now also U19.73, U20.5; no longer U28.73, U29.5
- net QSPI_IO37: now also U19.80, U20.2; no longer U28.80, U29.2
- net QSPI_IO38: now also U19.81, U20.3; no longer U28.81, U29.3
- net QSPI_IO39: now also U19.67, U20.7; no longer U28.67, U29.7
- net QSPI_IO4: now also U3.73, U4.5; no longer U4.73, U5.5
- net QSPI_IO40: now also U21.73, U22.5; no longer U31.73, U32.5
- net QSPI_IO41: now also U21.80, U22.2; no longer U31.80, U32.2
- net QSPI_IO42: now also U21.81, U22.3; no longer U31.81, U32.3
- net QSPI_IO43: now also U21.67, U22.7; no longer U31.67, U32.7
- net QSPI_IO44: now also U23.73, U24.5; no longer U34.73, U35.5
- net QSPI_IO45: now also U23.80, U24.2; no longer U34.80, U35.2
- net QSPI_IO46: now also U23.81, U24.3; no longer U34.81, U35.3
- net QSPI_IO47: now also U23.67, U24.7; no longer U34.67, U35.7
- net QSPI_IO48: now also U25.73, U26.5; no longer U37.73, U38.5
- net QSPI_IO49: now also U25.80, U26.2; no longer U37.80, U38.2
- net QSPI_IO5: now also U3.80, U4.2; no longer U4.80, U5.2
- net QSPI_IO50: now also U25.81, U26.3; no longer U37.81, U38.3
- net QSPI_IO51: now also U25.67, U26.7; no longer U37.67, U38.7
- net QSPI_IO52: now also U27.73, U28.5; no longer U40.73, U41.5
- net QSPI_IO53: now also U27.80, U28.2; no longer U40.80, U41.2
- net QSPI_IO54: now also U27.81, U28.3; no longer U40.81, U41.3
- net QSPI_IO55: now also U27.67, U28.7; no longer U40.67, U41.7
- net QSPI_IO56: now also U29.73, U30.5; no longer U43.73, U44.5
- net QSPI_IO57: now also U29.80, U30.2; no longer U43.80, U44.2
- net QSPI_IO58: now also U29.81, U30.3; no longer U43.81, U44.3
- net QSPI_IO59: now also U29.67, U30.7; no longer U43.67, U44.7
- net QSPI_IO6: now also U3.81, U4.3; no longer U4.81, U5.3
- net QSPI_IO60: now also U31.73, U32.5; no longer U46.73, U47.5
- net QSPI_IO61: now also U31.80, U32.2; no longer U46.80, U47.2
- net QSPI_IO62: now also U31.81, U32.3; no longer U46.81, U47.3
- net QSPI_IO63: now also U31.67, U32.7; no longer U46.67, U47.7
- net QSPI_IO7: now also U3.67, U4.7; no longer U4.67, U5.7
- net QSPI_IO8: now also U5.73, U6.5; no longer U7.73, U8.5
- net QSPI_IO9: now also U5.80, U6.2; no longer U7.80, U8.2
- net RX1/DEV_TX10: now also U19.28; no longer U28.28
- net RX1/DEV_TX11: now also U21.28; no longer U31.28
- net RX1/DEV_TX12: now also U23.28; no longer U34.28
- net RX1/DEV_TX13: now also U25.28; no longer U37.28
- net RX1/DEV_TX14: now also U27.28; no longer U40.28
- net RX1/DEV_TX15: now also U29.28; no longer U43.28
- net RX1/DEV_TX16: now also U31.28; no longer U46.28
- net RX1/DEV_TX2: now also U3.28; no longer U4.28
- net RX1/DEV_TX3: now also U5.28; no longer U7.28
- net RX1/DEV_TX4: now also U7.28; no longer U10.28
- net RX1/DEV_TX5: now also U9.28; no longer U13.28
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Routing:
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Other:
- outline, holes or cut-outs redrawn
